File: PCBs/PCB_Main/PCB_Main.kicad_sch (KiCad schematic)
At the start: 50 parts, among them J1 LED Connectors+, J2 To_Audio, J4 USB_B_Micro, J5 LED connectors -, J6 XT60-M, J7 HUB75, Q1 S8050, Q2 S8050, SW1 SW_Push, SW2 SW_Push, U1 CP2102N-Axx-xQFN28, U2 AMS1117-3.3, U3 ESP32-WROOM-E, U4 PCM5102A, U6 ESP32-WROVER-E

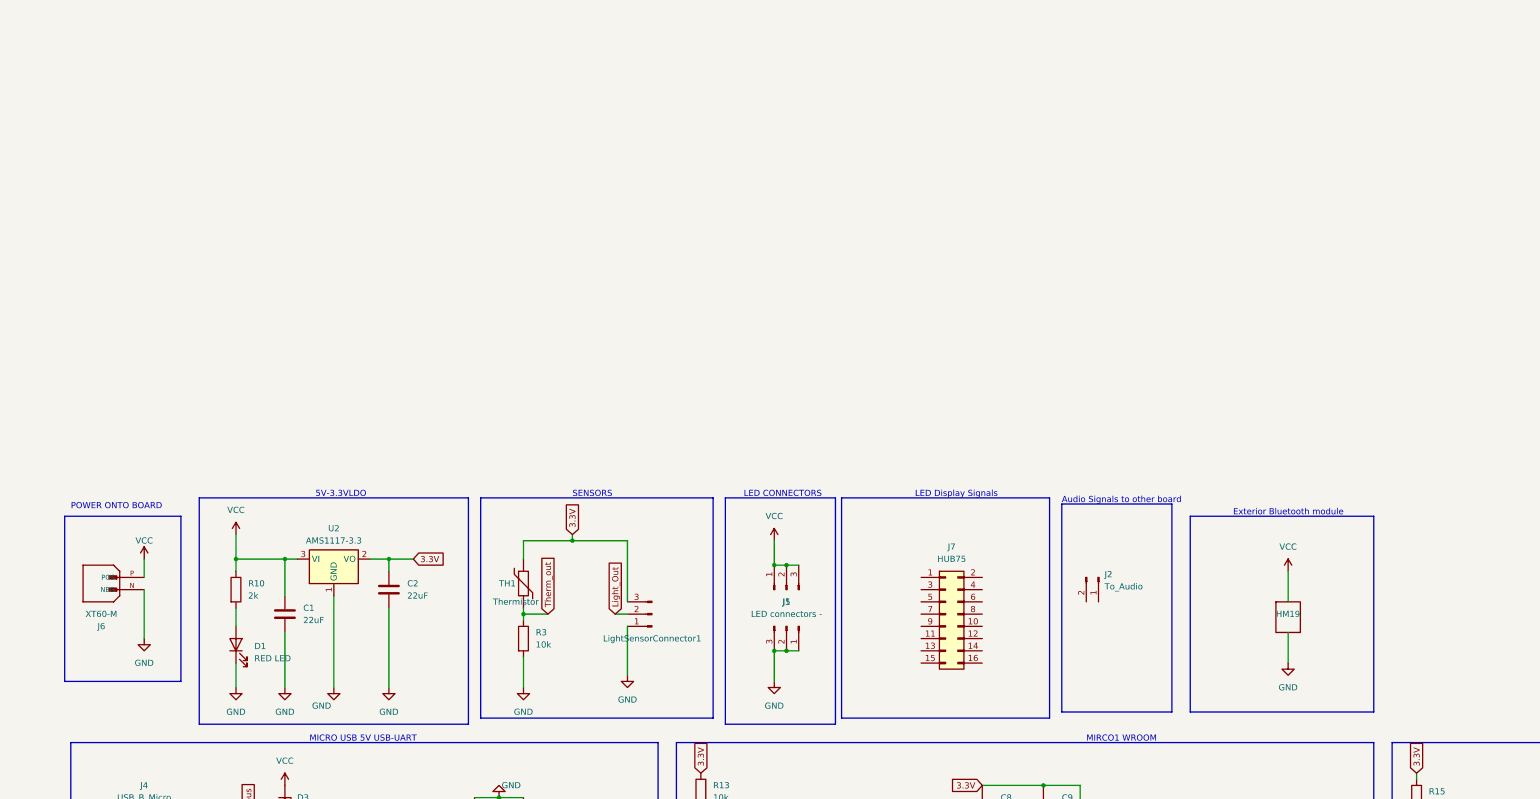
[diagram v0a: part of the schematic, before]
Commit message: PCB combination
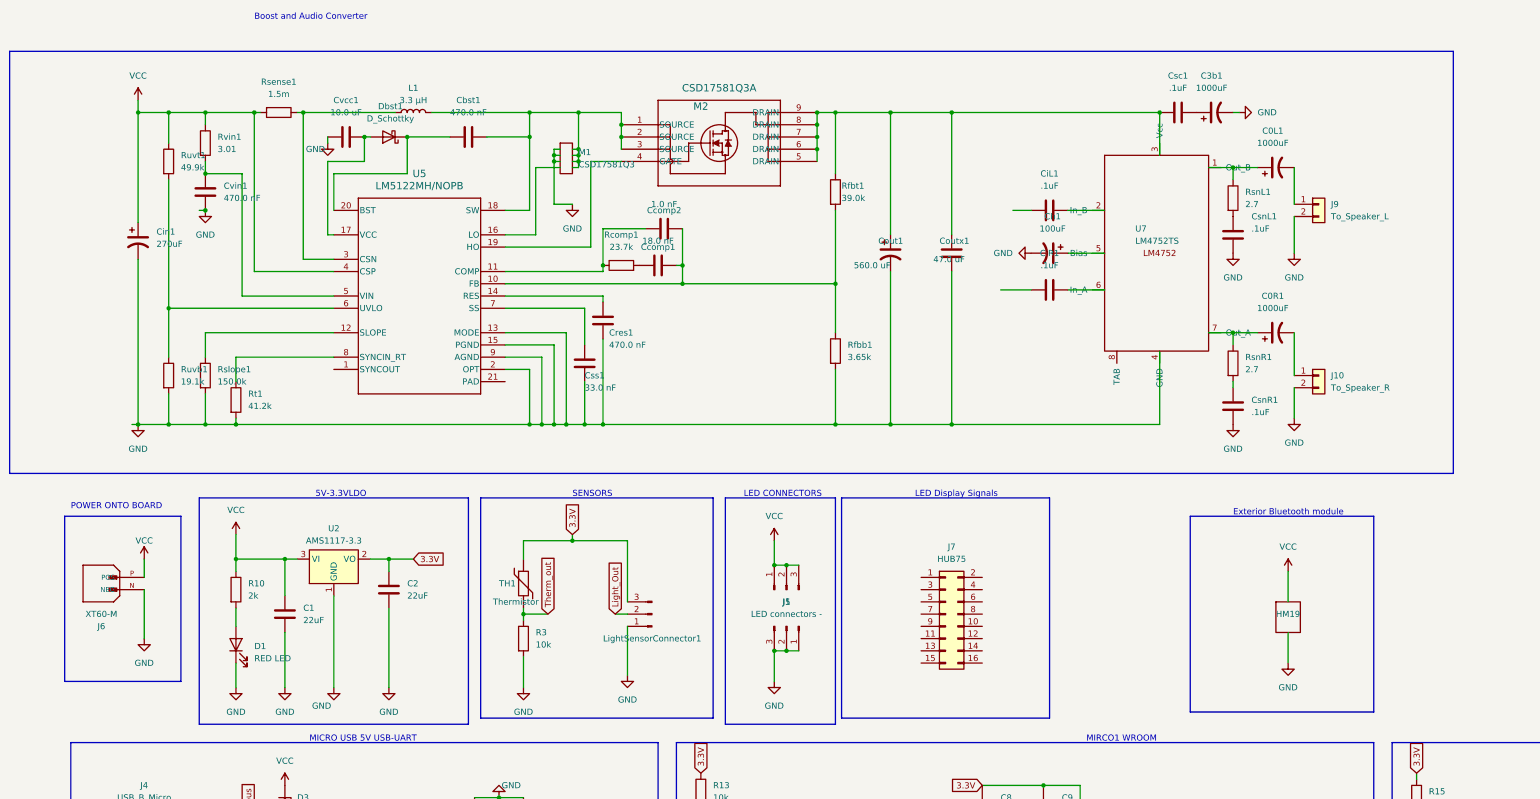
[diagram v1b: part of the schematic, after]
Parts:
- removed J2: To_Audio, Connector_PinHeader_2.54mm:PinHeader_1x02_P2.54mm_Vertical, symbol Connector:Conn_01x02_Pin
- added C0L1, C0R1, C3b1: 1000uF, Artisyn_Components:Audio_1000uF, symbol Device:C_Polarized_US
- added Cb1: 100uF, Artisyn_Components:Audio_100uF, symbol Device:C_Polarized_US
- added Cbst1, Cres1, Cvin1: 470.0 nF, Capacitor_SMD:C_0805_2012Metric, symbol Device:C
- added Ccomp1: 18.0 nF, Capacitor_SMD:C_1812_4532Metric, symbol Device:C
- added Ccomp2: 1.0 nF, Capacitor_SMD:C_0805_2012Metric, symbol Device:C
- added CiL1, CiR1, Csc1, CsnL1, CsnR1: .1uF, Capacitor_SMD:C_0805_2012Metric, symbol Device:C
- added Cin1: 270uF, Artisyn_Components:PCAP_SVP_E7_PAN, symbol Device:C_Polarized_US
- added Cout1: 560.0 uF, Artisyn_Components:PCAP_SVP_F12_PAN, symbol Device:C_Polarized_US
- added Coutx1: 47.0 uF, Capacitor_SMD:C_1206_3216Metric, symbol Device:C
- added Css1: 33.0 nF, Capacitor_SMD:C_0805_2012Metric, symbol Device:C
- added Cvcc1: 10.0 uF, Capacitor_SMD:C_0805_2012Metric, symbol Device:C
- added Dbst1: D_Schottky, Diode_SMD:D_SMA, symbol Device:D_Schottky
- added J10: To_Speaker_R, Connector_PinHeader_2.54mm:PinHeader_1x02_P2.54mm_Vertical, symbol Connector_Generic:Conn_01x02
- added J9: To_Speaker_L, Connector_PinHeader_2.54mm:PinHeader_1x02_P2.54mm_Vertical, symbol Connector_Generic:Conn_01x02
- added L1: 3.3 µH, Artisyn_Components:IND_R3-R_EAT, symbol Device:L
- added M1: CSD17581Q3, Artisyn_Components:CSD17309Q3, symbol Custom_Lib:CSD17309Q3
- added M2: CSD17581Q3A, Artisyn_Components:CSD17309Q3A, symbol CSD17581Q3A:CSD17581Q3A
- added Rcomp1: 23.7k, Resistor_SMD:R_0805_2012Metric, symbol Device:R
- added Rfbb1: 3.65k, Resistor_SMD:R_0805_2012Metric, symbol Device:R
- added Rfbt1: 39.0k, Resistor_SMD:R_0805_2012Metric, symbol Device:R
- added Rsense1: 1.5m, Resistor_SMD:R_2512_6332Metric, symbol Device:R
- added Rslope1: 150.0k, Resistor_SMD:R_0805_2012Metric, symbol Device:R
- added RsnL1, RsnR1: 2.7, Resistor_SMD:R_0805_2012Metric, symbol Device:R
- added Rt1: 41.2k, Resistor_SMD:R_0805_2012Metric, symbol Device:R
- added Ruvb1: 19.1k, Resistor_SMD:R_0805_2012Metric, symbol Device:R
- added Ruvt1: 49.9k, Resistor_SMD:R_0805_2012Metric, symbol Device:R
- added Rvin1: 3.01, Resistor_SMD:R_1206_3216Metric, symbol Device:R
- added U5: LM5122MH/NOPB, Artisyn_Components:LM512220A_L, symbol LM5122:LM5122MH_NOPB
- added U7: LM4752TS, Artisyn_Components:LM4752, symbol LM4752TS:LM4752TS
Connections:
- net GND: now also C3b1.2, Cb1.2, Cin1.2, Cout1.2, Coutx1.2, Cres1.2, CsnL1.2, CsnR1.2, Css1.2, Cvcc1.1, Cvin1.2, J10.2 (Pin_2), J9.2 (Pin_2), M1.1 (S1), M1.2 (S2), M1.3 (S3), Rfbb1.2, Rslope1.2, Rt1.2, Ruvb1.2, U5.13 (MODE), U5.15 (PGND), U5.2 (OPT), U5.9 (AGND), U7.4 (GND)
- net VCC: now also Cin1.1, Rsense1.2, Ruvt1.1, Rvin1.1, U5.4 (CSP)
- new net: CiL1.2, U7.2 (In_B)
- new net: Cvcc1.2, Dbst1.2 (A), U5.17 (VCC)
- new net: Ccomp2.1, Rcomp1.1, U5.11 (COMP)
- new net: Ccomp1.2, Ccomp2.2, Rfbb1.1, Rfbt1.2, U5.10 (FB)
- new net: Cout1.1, Coutx1.1, Csc1.1, M2.5 (DRAIN), M2.6 (DRAIN), M2.7 (DRAIN), M2.8 (DRAIN), M2.9 (DRAIN), Rfbt1.1, U7.3 (Vcc)
- new net: C0R1.1, RsnR1.1, U7.7 (Out_A)
- new net: C0R1.2, J10.1 (Pin_1)
- new net: C0L1.1, RsnL1.1, U7.1 (Out_B)
- new net: CsnL1.1, RsnL1.2
- new net: Cb1.1, U7.5 (Bias)
- new net: CiR1.2, U7.6 (In_A)
- new net: C3b1.1, Csc1.2
- new net: Ccomp1.1, Rcomp1.2
- new net: Rt1.1, U5.8 (SYNCIN_RT)
- new net: Cbst1.2, L1.2, M1.5 (D1), M1.6 (D2), M1.7 (D3), M1.8 (D4), M2.1 (SOURCE), M2.2 (SOURCE), M2.3 (SOURCE), U5.18 (SW)
- new net: M2.4 (GATE), U5.19 (HO)
- new net: Cvin1.1, Rvin1.2, U5.5 (VIN)
- new net: Rslope1.1, U5.12 (SLOPE)
- new net: L1.1, Rsense1.1, U5.3 (CSN)
- new net: CsnR1.1, RsnR1.2
- new net: Ruvb1.1, Ruvt1.2, U5.6 (UVLO)
- new net: C0L1.2, J9.1 (Pin_1)
- new net: Css1.1, U5.7 (SS)
- new net: Cres1.1, U5.14 (RES)
- new net: M1.4 (G), U5.16 (LO)
- new net: Cbst1.1, Dbst1.1 (K), U5.20 (BST)
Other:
- note added: "Boost and Audio Converter"
- note removed: "Audio Signals to other board"
